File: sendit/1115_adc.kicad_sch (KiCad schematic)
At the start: 5 parts, among them U7 ADS1115IDGSR

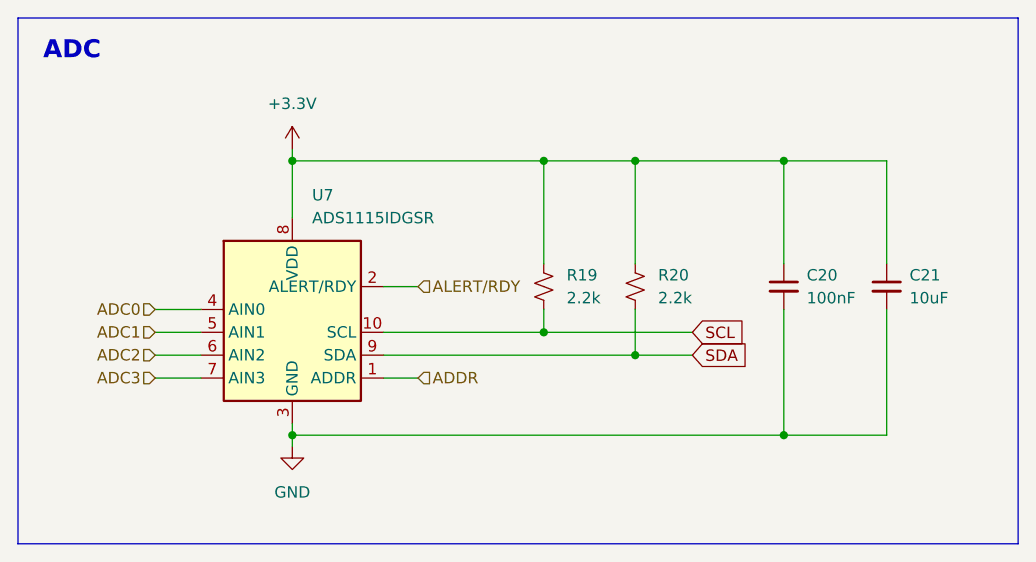
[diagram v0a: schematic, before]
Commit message: more work towards rev c board.
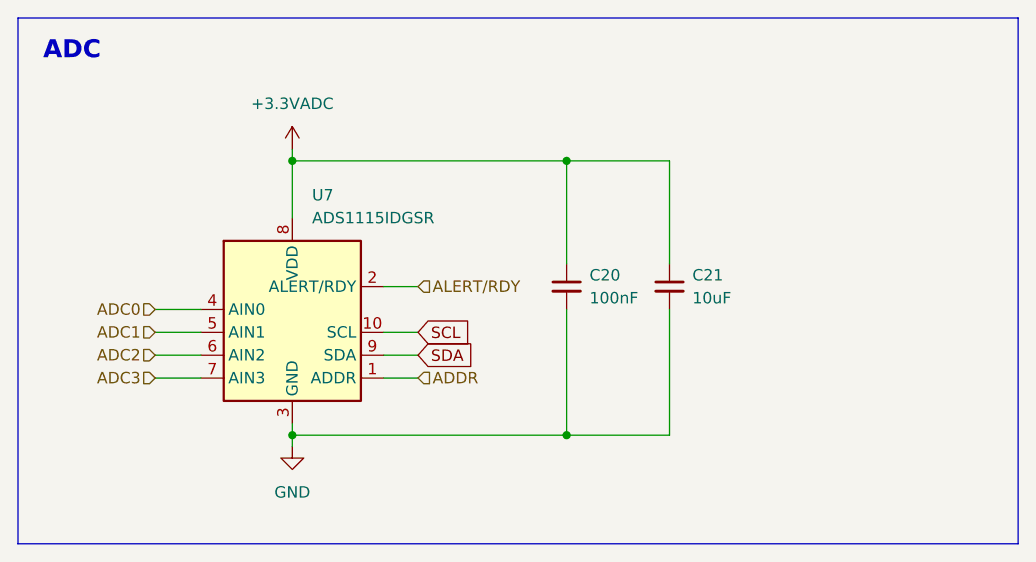
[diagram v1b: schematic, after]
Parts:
- removed R19, R20: 2.2k, Resistor_SMD:R_0603_1608Metric, symbol Device:R_Small_US
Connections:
- net +3.3V renamed +3.3VADC
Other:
- moved on the sheet: C20, C21
